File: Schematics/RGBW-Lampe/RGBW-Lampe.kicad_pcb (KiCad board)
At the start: 2 copper layers, 99.6 x 69.6 mm, 142 parts, among them J1 Conn_01x10, J2 Conn_01x04, J3 Conn_01x08, J4 Conn_01x02, J5 Conn_01x04_Male, J6 Conn_02x05_Odd_Even, J7 Conn_01x02, J8 Conn_01x02, Q1 BSS138, Q2 BSS138, Q3 BSS138, Q4 BSS138, T1 SFH320, U1 LIS2DH, U2 ESP-12F, U3 L5973D, U4 24LC16, U5 TSOP348xx, U6 TDA7052A, U7 STM32L151CBTx, Y1 12MHz, Y2 32,768 MS1V 7

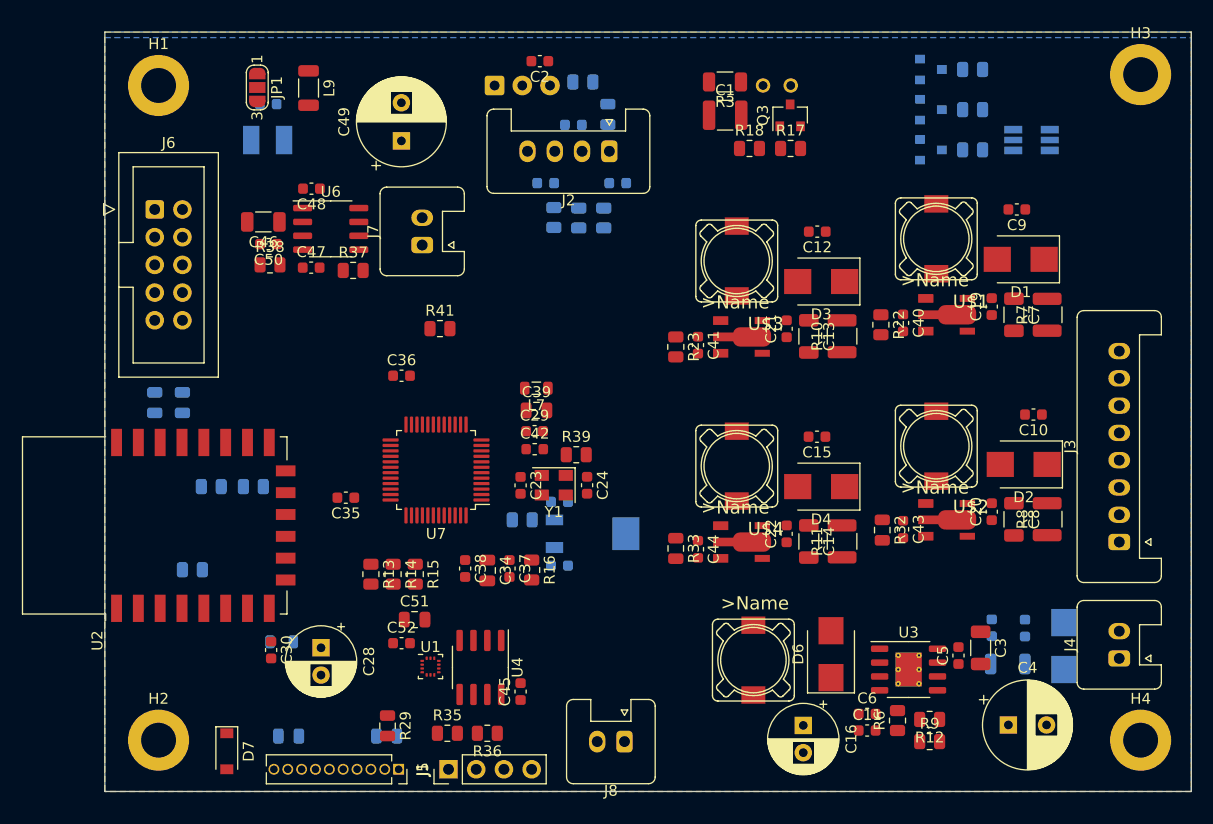
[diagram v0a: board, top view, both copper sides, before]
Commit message: PCB version produced
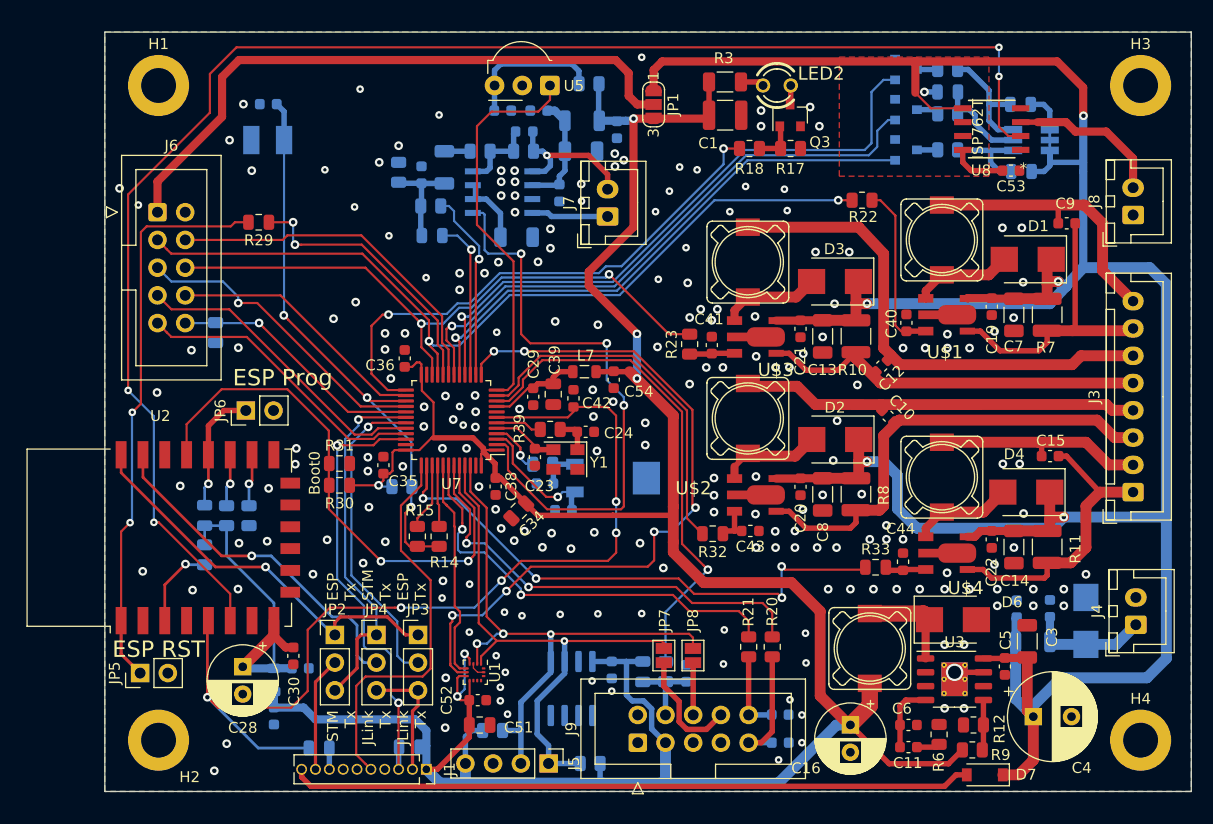
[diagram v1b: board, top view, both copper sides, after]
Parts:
- removed J2: Conn_01x04, Connector_Stocko:Stocko_MKS_1654-6-0-404_1x4_P2.50mm_Vertical
- added C53: 220nF / 25V, Capacitor_SMD:C_0603_1608Metric, F.Cu at (183.1, 82.8)
- added C54: 10n, Capacitor_SMD:C_0603_1608Metric, F.Cu at (146.7, 102.0)
- added C55: 10n, Capacitor_SMD:C_0603_1608Metric, B.Cu at (115.6, 132.8)
- added C56: 10n, Capacitor_SMD:C_0603_1608Metric, B.Cu at (118.0, 128.4)
- added C57: 10n, Capacitor_SMD:C_0603_1608Metric, B.Cu at (147.0, 79.1)
- added C58: 10n, Capacitor_SMD:C_0603_1608Metric, B.Cu at (139.8, 77.3)
- added J9: Conn_02x05_Odd_Even, Connector_IDC:IDC-Header_2x05_P2.54mm_Vertical, F.Cu at (148.9, 135.2)
- added JP2: Jumper_3_Open, Connector_PinHeader_2.54mm:PinHeader_1x03_P2.54mm_Vertical, F.Cu at (121.2, 125.3)
- added JP3: Jumper_3_Open, Connector_PinHeader_2.54mm:PinHeader_1x03_P2.54mm_Vertical, F.Cu at (128.8, 125.3)
- added JP4: Jumper_3_Open, Connector_PinHeader_2.54mm:PinHeader_1x03_P2.54mm_Vertical, F.Cu at (125.0, 125.3)
- added JP5: Jumper_2_Open, Connector_PinHeader_2.54mm:PinHeader_1x02_P2.54mm_Vertical, F.Cu at (103.3, 128.8)
- added JP6: Jumper_2_Open, Connector_PinHeader_2.54mm:PinHeader_1x02_P2.54mm_Vertical, F.Cu at (113.0, 104.8)
- added JP7: SolderJumper_2_Open, Jumper:SolderJumper-2_P1.3mm_Open_Pad1.0x1.5mm, F.Cu at (151.3, 127.2)
- added JP8: SolderJumper_2_Open, Jumper:SolderJumper-2_P1.3mm_Open_Pad1.0x1.5mm, F.Cu at (154.0, 127.2)
- added R42: 10k, Resistor_SMD:R_0805_2012Metric, B.Cu at (109.2, 114.4)
- added R43: 180, Resistor_SMD:R_0805_2012Metric, B.Cu at (130.1, 88.8)
- added R44: 1.2k, Resistor_SMD:R_0805_2012Metric, B.Cu at (127.0, 83.0)
- added R45: ob, Resistor_SMD:R_0805_2012Metric, B.Cu at (184.0, 76.7)
- added R46: ob, Resistor_SMD:R_0805_2012Metric, B.Cu at (184.1, 82.9)
- added R47: ob, Resistor_SMD:R_0805_2012Metric, B.Cu at (177.3, 75.6)
- added U8: ISP762T, ISP762:ISP762T, F.Cu at (181.4, 79.0)
- C2, C45, C46, C48, C50, L9, R13, R35, R36, R41, U4: moved to B.Cu
- C37: value 220n -> 1µF / 50V X7R; footprint Capacitor_SMD:C_0603_1608Metric -> Capacitor_SMD:C_1206_3216Metric; moved to B.Cu
- C47: value 220nF / 25V -> 100µF / 6,3V; footprint Capacitor_SMD:C_0603_1608Metric -> Capacitor_SMD:C_1206_3216Metric; moved to B.Cu
- C49: value 470µF / 25V -> 1n; footprint Capacitor_THT:CP_Radial_D8.0mm_P3.50mm -> Capacitor_SMD:C_0603_1608Metric; moved to B.Cu
- J3: footprint Connector_Stocko:Stocko_MKS_1658-6-0-808_1x8_P2.50mm_Vertical -> Connector_JST:JST_XH_B8B-XH-A_1x08_P2.50mm_Vertical
- J4, J7, J8: footprint Connector_Stocko:Stocko_MKS_1652-6-0-202_1x2_P2.50mm_Vertical -> Connector_JST:JST_XH_B2B-XH-A_1x02_P2.50mm_Vertical
- L7, L8: value BLM18 -> BLM21PG 331
- LED2, R20, R21, R30, R31, U5: moved to F.Cu
- R10, R11, R7, R8: value 0.2 -> 0.150
- R16, R37: value 100 -> 22k; moved to B.Cu
- R38: value 100 -> 1.2k; moved to B.Cu
- U6: value TDA7052A -> LM4861M; footprint Package_SO:SO-8_3.9x4.9mm_P1.27mm -> LM4861:LM4861M; moved to B.Cu
- moved D7 69.5 mm to (180.7, 138.2), turned to 180 degrees
- moved J8 67.1 mm to (194.3, 86.9), turned to 90 degrees
- moved C33 59.7 mm to (162.0, 135.2), turned to 0 degrees
- moved C32 53.2 mm to (162.0, 132.7), turned to 0 degrees
- moved R26 51.2 mm to (149.4, 128.7)
- moved R29 47.6 mm to (114.2, 87.5), turned to 180 degrees
- moved C31 45.4 mm to (153.4, 128.9), turned to 90 degrees
- moved R21 43.2 mm to (159.1, 126.4), turned to 90 degrees
- moved R20 43.1 mm to (161.2, 126.4), turned to 90 degrees
- moved R19 42.0 mm to (151.5, 128.7), turned to 90 degrees
- moved R16 38.4 mm to (138.5, 81.0), turned to 180 degrees
- moved JP1 36.4 mm to (150.4, 76.7)
- moved C37 30.4 mm to (137.8, 88.9), turned to 0 degrees
- moved C47 26.9 mm to (143.7, 81.0)
- moved L9 25.2 mm to (143.8, 78.2), turned to 180 degrees
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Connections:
- C1 pad 1: +12V -> +3V3
- C47 pad 1: GND -> Net-(C47-Pad1)
- C47 pad 2: Net-(C47-Pad2) -> GND
- C48 pad 1: Net-(C48-Pad1) -> GND
- C48 pad 2: Net-(C48-Pad2) -> Net-(C47-Pad1)
- C49 pad 1: Net-(C48-Pad2) -> Net-(C49-Pad1)
- D6 pad 1: GND -> Net-(D6-Pad1)
- D6 pad 2: Net-(D6-Pad2) -> GND
- J1 pad 2: Net-(J1-Pad2) -> /Control/J-Link_TX
- J1 pad 9: /Control/USART1_TX -> /Control/J-Link_RX
- J7 pad 2: Net-(J7-Pad2) -> Net-(C49-Pad2)
- J8 pad 1: Net-(J8-Pad1) -> GND
- J8 pad 2: GND -> Net-(J8-Pad2)
- L6 pad P$1: Net-(D6-Pad2) -> Net-(D6-Pad1)
- L9 pad 1: +12VA -> +3V3
- L9 pad 2: Net-(C48-Pad2) -> Net-(C47-Pad1)
- R16 pad 1: Net-(C37-Pad1) -> Net-(C49-Pad2)
- R16 pad 2: Net-(J8-Pad1) -> Net-(C49-Pad1)
- R22 pad 1: LED_1_PWM -> LED_3_PWM
- R23 pad 1: LED_2_PWM -> LED_4_PWM
- R29 pad 1: /Control/USART1_RX -> /Control/ESP_RST
- R29 pad 2: Net-(J1-Pad2) -> Net-(JP5-Pad1)
- R3 pad 2: +12V -> +3V3
- R32 pad 1: LED_3_PWM -> LED_1_PWM
- R33 pad 1: LED_4_PWM -> LED_2_PWM
- R37 pad 1: Net-(C47-Pad2) -> Net-(C49-Pad1)
- R37 pad 2: Volume -> Net-(C46-Pad1)
- U2 pad 1: /Control/ESP_RST -> Net-(JP5-Pad1)
- U2 pad 18: /Control/ESP_GPIO_0 -> Net-(JP6-Pad1)
- U2 pad 21: /Control/USART1_TX -> /Control/ESP_RX
- U2 pad 22: /Control/USART1_RX -> /Control/ESP_TX
- U2 pad 6: Net-(U2-Pad6) -> ExtPower
- U3 pad 1: Net-(D6-Pad2) -> Net-(D6-Pad1)
- U6 pad 1: Net-(C48-Pad2) -> AMP_SHTDN
- U6 pad 2: Net-(C46-Pad1) -> Net-(C37-Pad1)
- U6 pad 3: GND -> Net-(C37-Pad1)
- U6 pad 4: Net-(C47-Pad2) -> Net-(C49-Pad1)
- U6 pad 5: Net-(J7-Pad1) -> Net-(C49-Pad2)
- U6 pad 6: GND -> Net-(C47-Pad1)
- U6 pad 7: Net-(U6-Pad7) -> GND
- U6 pad 8: Net-(J7-Pad2) -> Net-(J7-Pad1)
- U7 pad 1: Net-(C37-Pad1) -> +3V3
- U7 pad 19: /Control/LCD_Backlight_PWM -> /Control/LCD_BACKLIGHT_PWM
- U7 pad 2: /Control/ESP_GPIO_0 -> AMP_SHTDN
- U7 pad 30: /Control/USART1_TX -> /Control/STM32_TX
- U7 pad 31: /Control/USART1_RX -> /Control/STM32_RX
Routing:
- net +12V: track 0.00 -> 273.4 mm, vias 0 -> 6
- net +3V3: track 0.00 -> 267.4 mm, vias 0 -> 6
- net ExtPower: track 0.00 -> 140.3 mm, vias 0 -> 4
- net /Control/NRST: track 0.00 -> 89.8 mm, vias 0 -> 5
- net LED_3_PWM: track 0.00 -> 77.7 mm, vias 0 -> 2
- net /Control/INT1: track 0.00 -> 66.5 mm, vias 0 -> 6
- net Net-(D7-Pad2): track 0.00 -> 62.5 mm
- net Net-(J6-Pad1): track 0.00 -> 57.9 mm
- net LED_4_PWM: track 0.00 -> 57.6 mm, vias 0 -> 2
- net /Control/STATUS_LED_R_PWM: track 0.00 -> 57.3 mm, vias 0 -> 1
- net AMP_SHTDN: track 0.00 -> 54.5 mm, vias 0 -> 3
- net /Control/SDA: track 0.00 -> 54.5 mm, vias 0 -> 3
- net /Control/STATUS_LED_B_PWM: track 0.00 -> 54.4 mm, vias 0 -> 1
- net Net-(JP5-Pad1): track 0.00 -> 53.2 mm, vias 0 -> 2
- net LED_2_PWM: track 0.00 -> 52.6 mm, vias 0 -> 4
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- added copper zone on F.Cu, net +12V
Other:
- net class Default: clearance 0.2 -> 0.1; trace_width 0.25 -> 0.1; via_dia 0.8 -> 0.7; via_drill 0.4 -> 0.3
- rule trace_clearance: 0.2 -> 0.1
- rule trace_min: 0.2 -> 0.1
- board text added: "Boot0"
- board text added: "ESP Prog"
- board text added: "ESP RST"
- board text added: "ESP Tx STM Tx ESP Tx"
- board text added: "STM Tx JLink Tx JLink Tx"

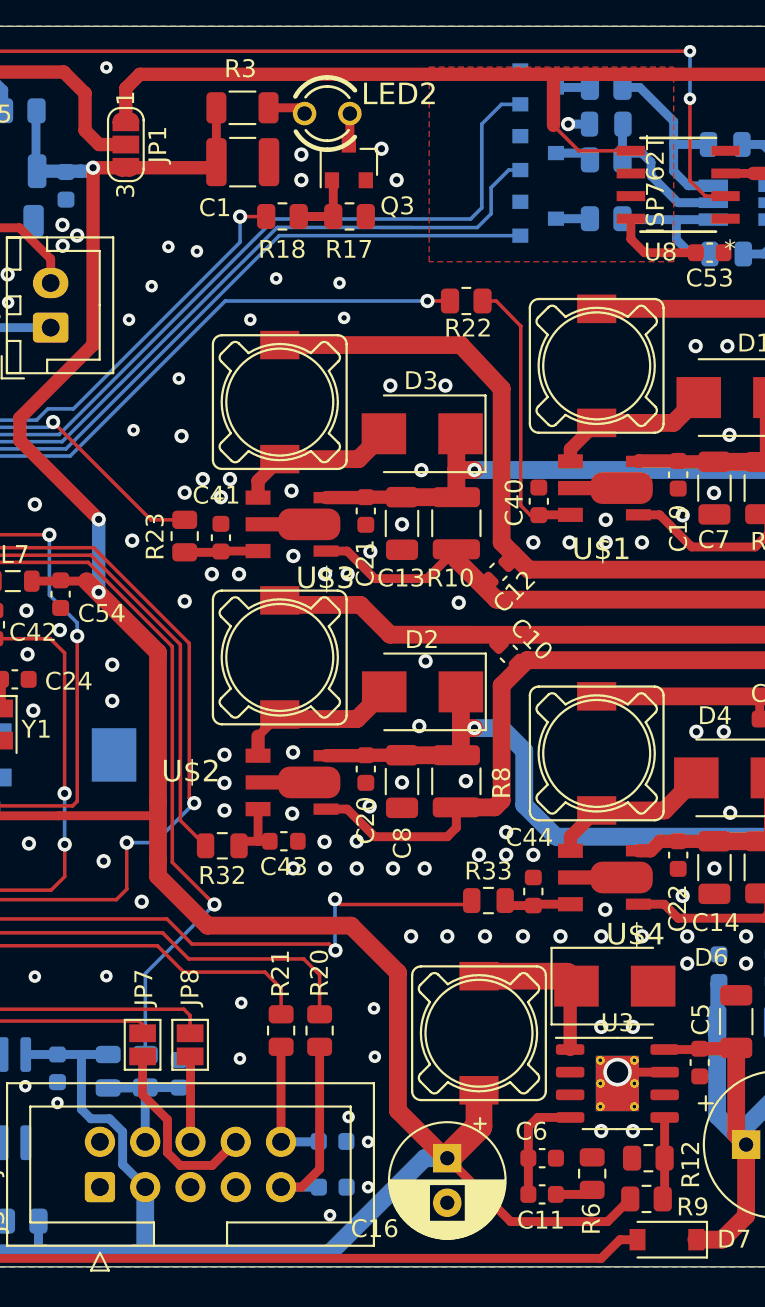
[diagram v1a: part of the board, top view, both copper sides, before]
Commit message: updated kicad version
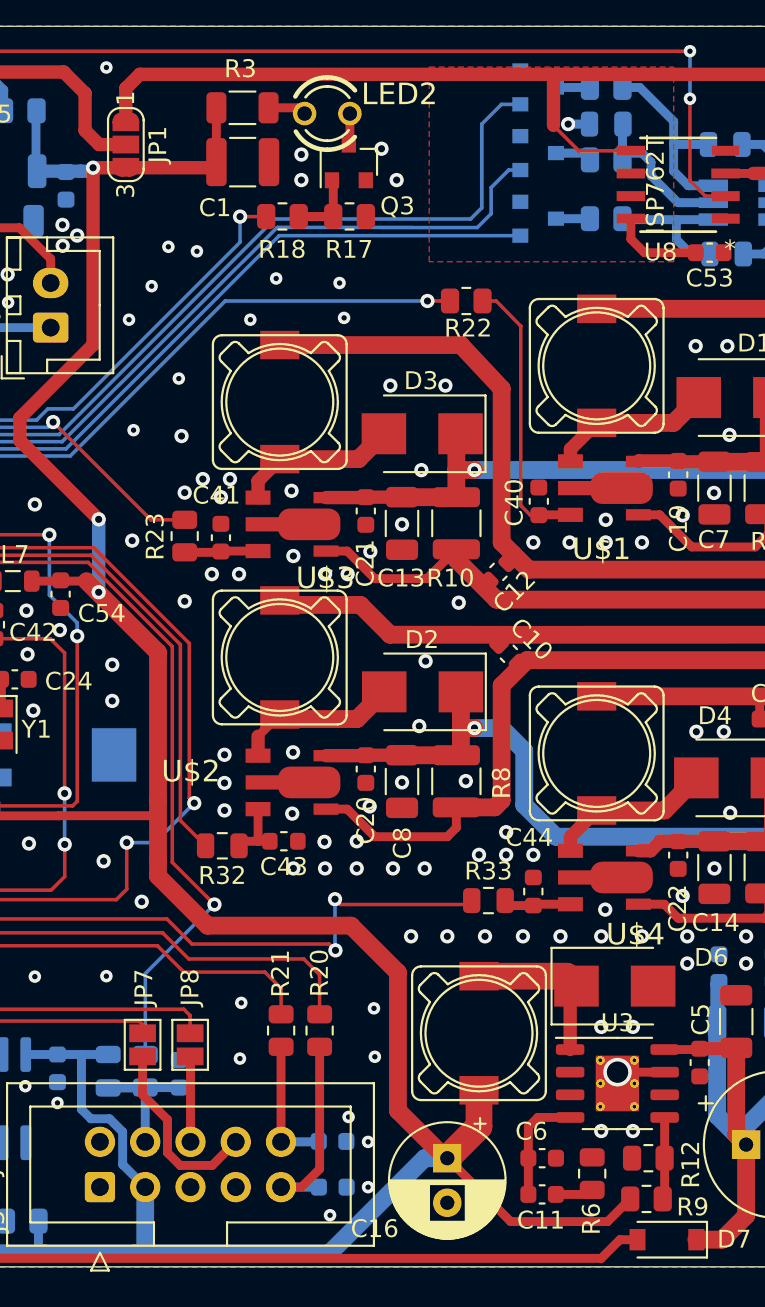
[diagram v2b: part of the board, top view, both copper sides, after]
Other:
- net class Default removed
